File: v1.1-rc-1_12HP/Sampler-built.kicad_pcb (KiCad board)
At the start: 4 copper layers, 241.5 x 109.2 mm, 231 parts, among them J10 Eurorack_Power_10pin_Unshroud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, J11 3.5mm_Mono_Switched, J12 3.5mm_Mono_Switched, J13 3.5mm_Mono_Switched, J14 3.5mm_Mono_Switched, J15 3.5mm_Mono_Switched, J16 3.5mm_Mono_Switched, J17 3.5mm_Mono_Switched, J2 3.5mm_Mono_Switched, J3 Conn_01x04, J4 Conn_02x04, J6 3.5mm_Mono_Switched, J7 3.5mm_Mono_Switched, J8 3.5mm_Mono_Switched, J9 3.5mm_Mono_Switched, U1 TL072H, U10 TL072H, U11 TL072H, U12 TL072H, U13 AP62200WU-7, U14 TL072H, U15 NJM2068, U16 NJM2068, U2 STM32F746IE, U3 TL072H, U4 SDRAM_IS42S16400J-6BLI-TR, U5 TL072H, U6 NCP51460SN33, U8 TL072H, U9 PCM3060PW, Y1 16MHz_18pF_FA238

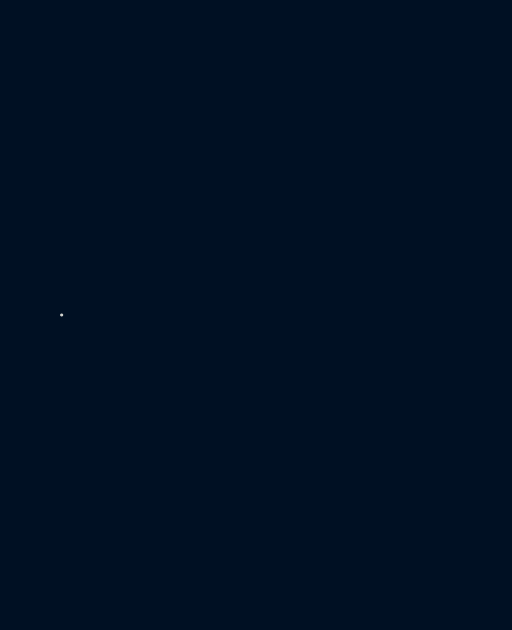
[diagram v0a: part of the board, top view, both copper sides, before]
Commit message: Removed extra EdgeCuts line
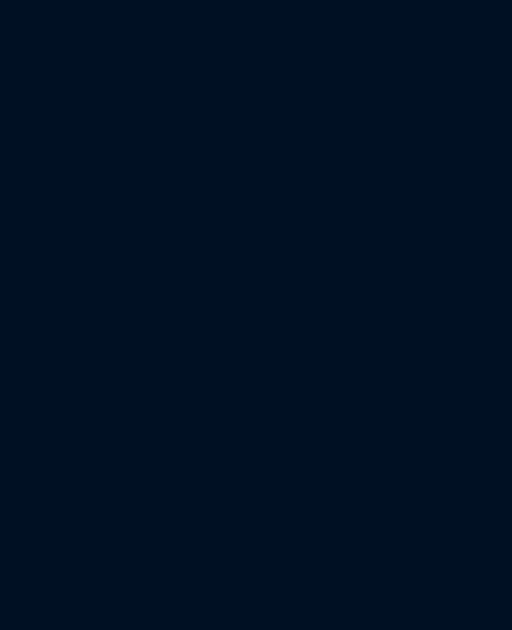
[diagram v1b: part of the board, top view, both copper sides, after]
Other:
- board size 241.5 x 109.2 mm -> 60.5 x 109.2 mm
